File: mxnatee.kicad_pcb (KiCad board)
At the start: 2 copper layers, 137.5 x 139.4 mm, 49 parts, among them U1 ProMicro, U2 TRRS, U4 HOLE

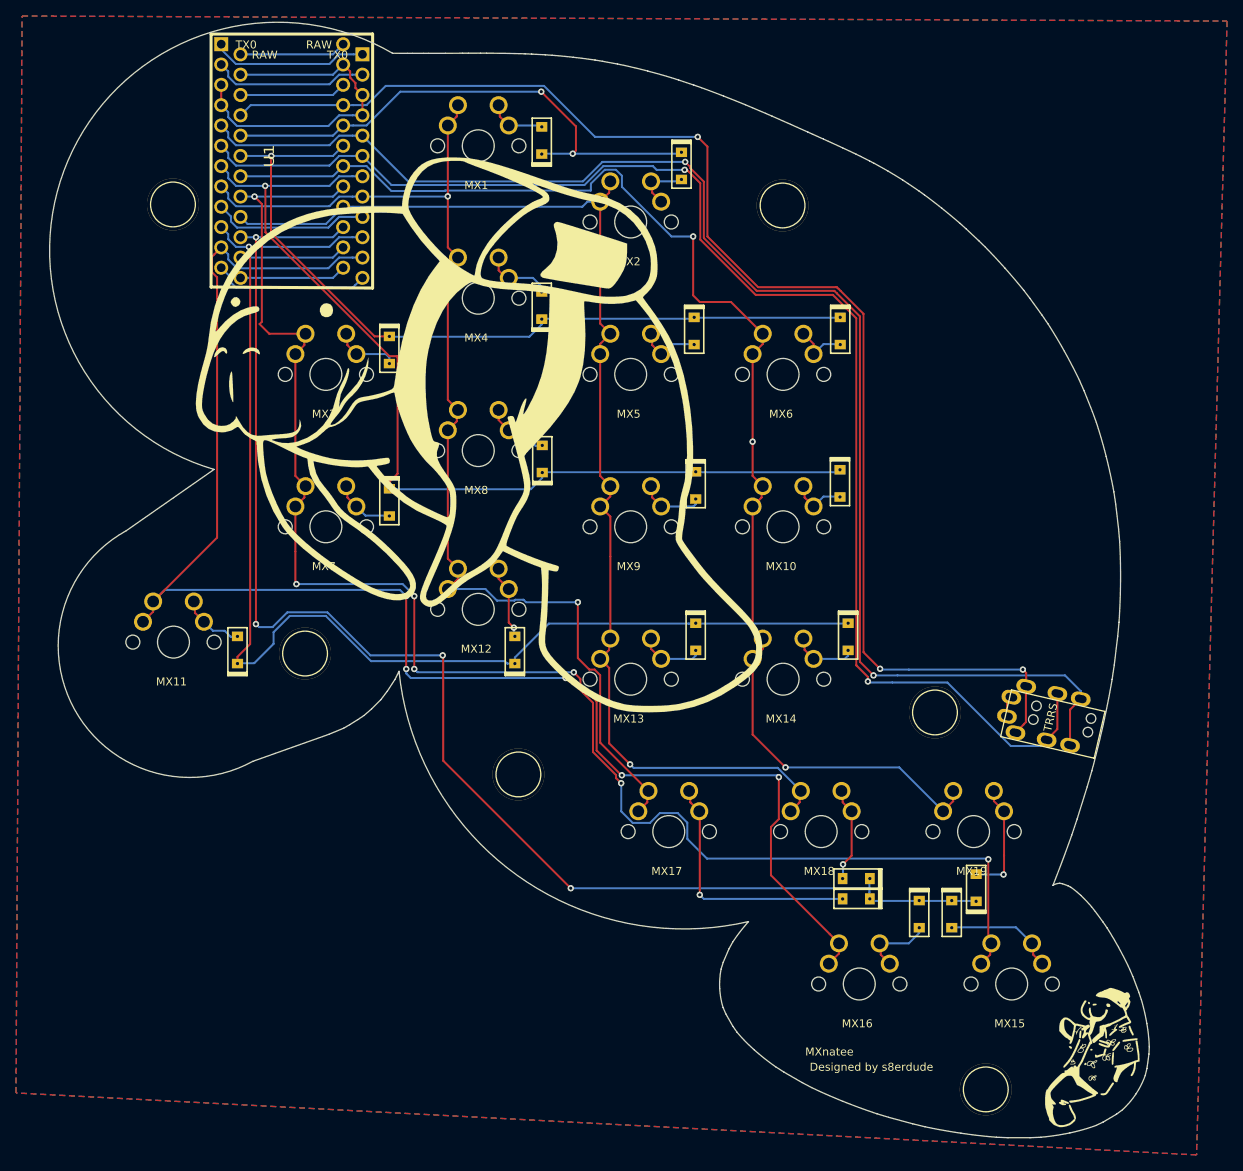
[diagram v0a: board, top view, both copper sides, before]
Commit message: Update
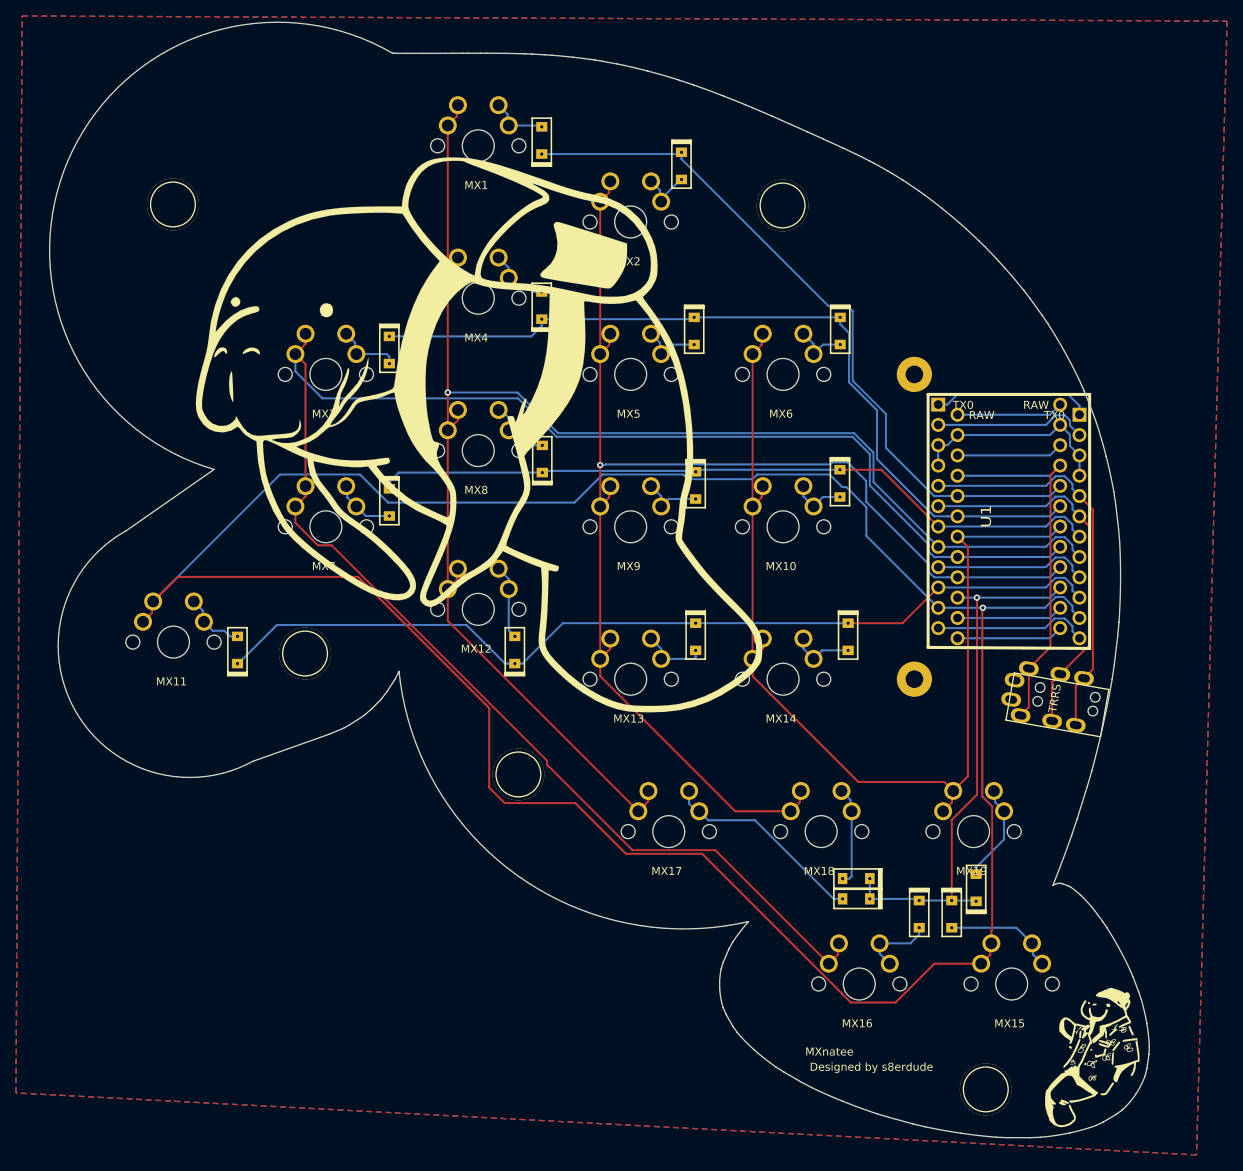
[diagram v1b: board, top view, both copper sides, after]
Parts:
- removed the U4 at (122.8, 98.4)
- added REF**: MountingHole_2.2mm_M2_Pad_NoSilk, Keybage_MountingHoles:MountingHole_2.2mm_M2_Pad_NoSilk, F.Cu at (120.2, 56.2)
- added REF**: MountingHole_2.2mm_M2_Pad_NoSilk, Keybage_MountingHoles:MountingHole_2.2mm_M2_Pad_NoSilk, F.Cu at (120.2, 94.3)
- moved U1 100.3 mm to (130.8, 73.9)
- moved U2 2.78 mm to (144.0, 98.5), turned to 260 degrees
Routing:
- net DATA2: track 176.9 -> 49.8 mm, vias 2 -> 0
- net DATA1: track 174.1 -> 47.5 mm, vias 2 -> 0
- net VCC: track 169.5 -> 46.6 mm, vias 3 -> 0
- net ROW4: track 177.3 -> 68.5 mm, vias 4 -> 1
- net COL0: track 217.5 -> 320.1 mm, vias 5 -> 1
- net COL2: track 142.5 -> 202.3 mm, vias 2 -> 1
- net COL1: track 176.5 -> 228.8 mm, vias 7 -> 0
- net ROW3: track 156.9 -> 115.2 mm, vias 1 -> 0
- net COL4: track 165.9 -> 130.0 mm, vias 3 -> 0
- net ROW2: track 123.0 -> 92.7 mm, vias 1 -> 0
- net ROW0: track 67.1 -> 91.3 mm, vias 2 -> 0
- net COL3: track 150.4 -> 172.0 mm
- net GND: track 45.5 -> 26.2 mm
- net Net-(D17-Pad2): track 31.7 -> 25.7 mm, vias 1 -> 0
- net ROW1: track 101.0 -> 103.9 mm, vias 1 -> 0
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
